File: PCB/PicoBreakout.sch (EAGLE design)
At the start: 41 parts

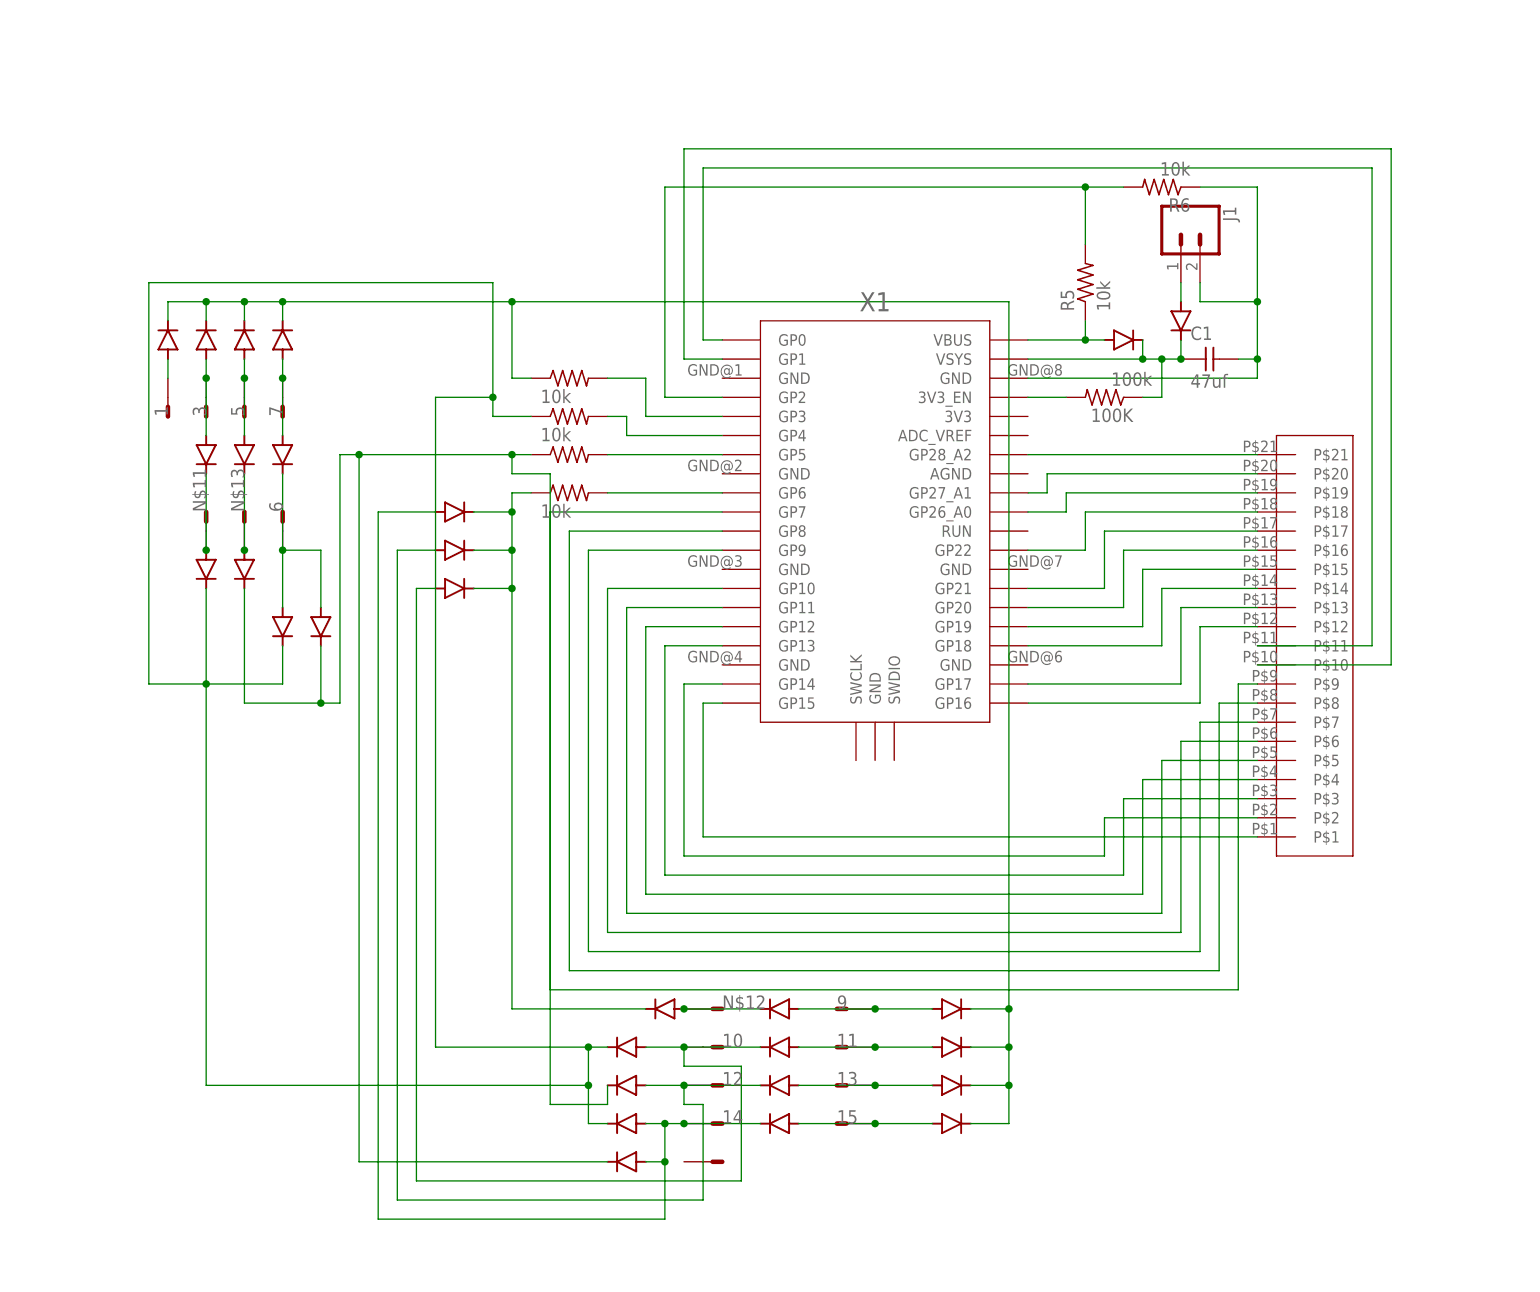
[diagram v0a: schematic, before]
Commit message: schematic push
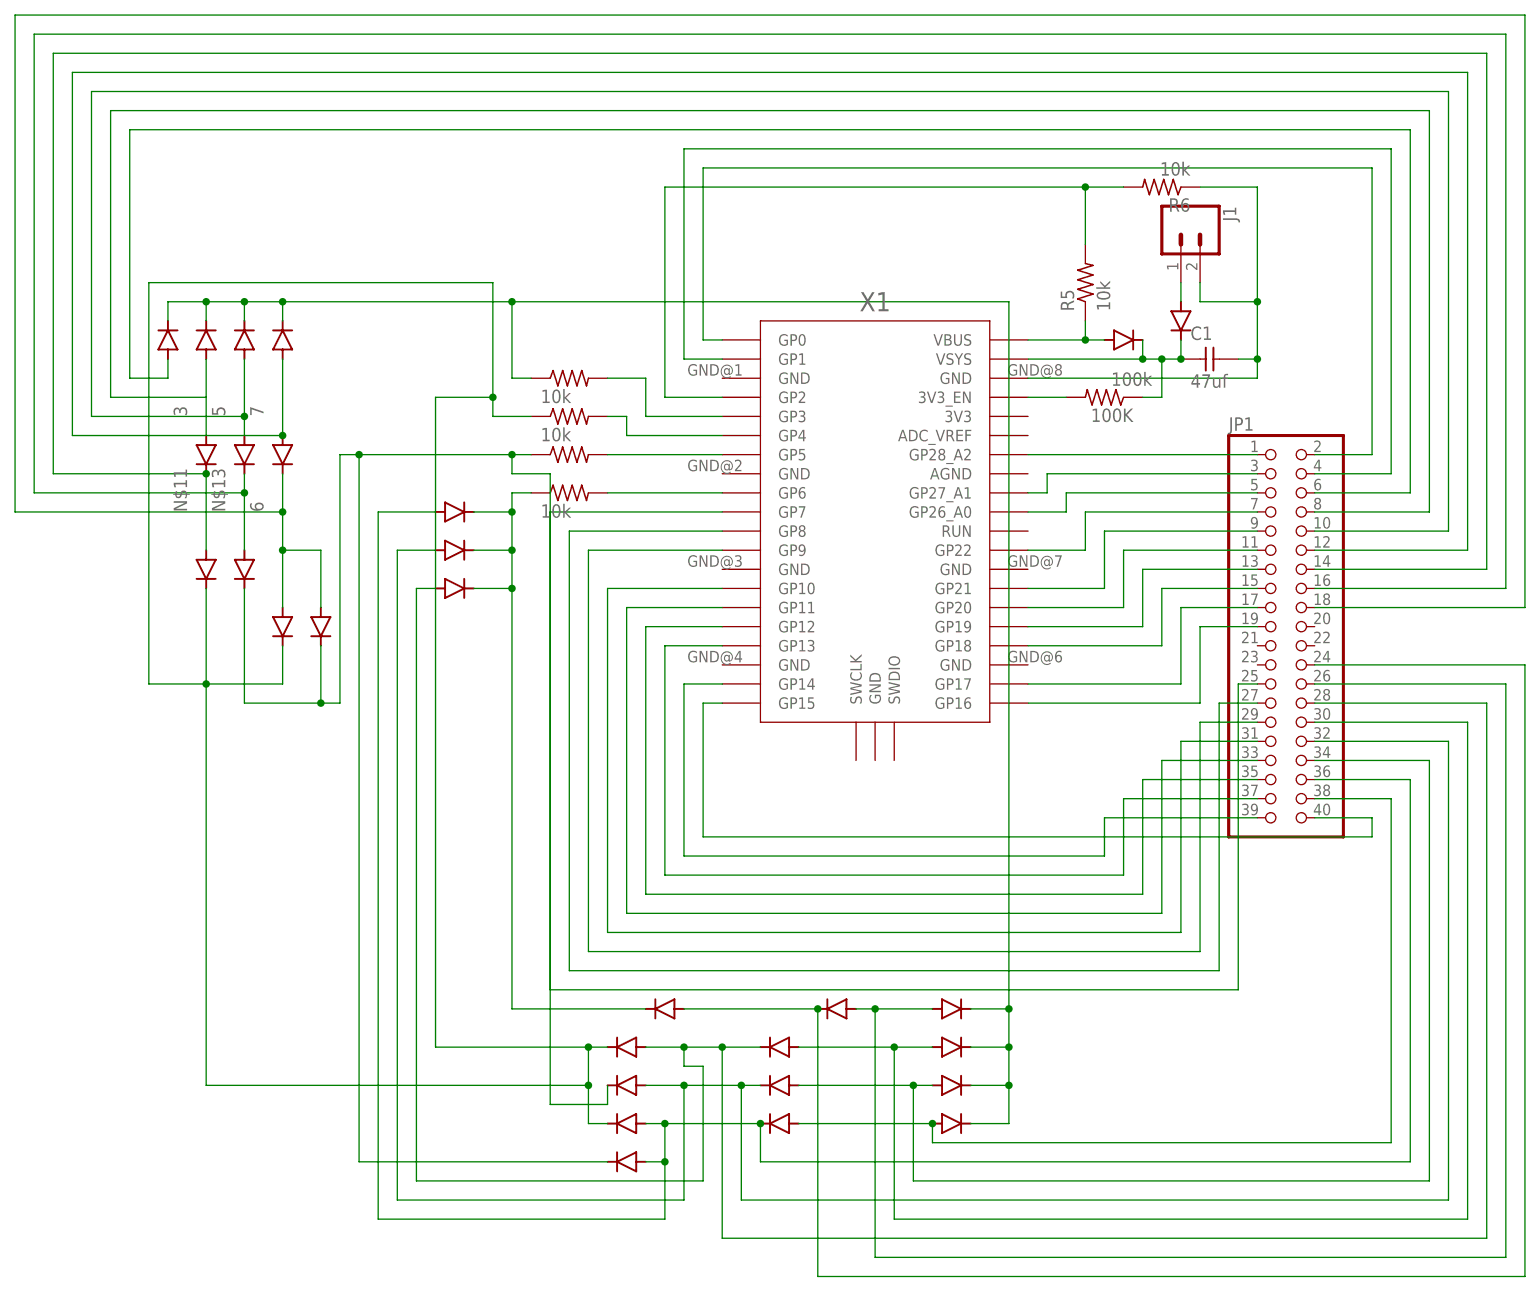
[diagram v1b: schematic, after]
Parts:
- removed SV1: (no value), con-dil:16E
- removed U$1: 21-SMD-CONN, ContunityTestingRig:21-SMD-CONN
- added JP1: (no value), adafruit:PINHD-2X20
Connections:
- net 10: now also JP1.28; no longer SV1-10.S
- net 11: now also JP1.30; no longer SV1-11.S
- net 12: now also JP1.32; no longer SV1-12.S
- net 13: now also JP1.34; no longer SV1-13.S
- net 14: now also JP1.36; no longer SV1-14.S
- net 15: now also JP1.38; no longer SV1-15.S
- net 3: now also JP1.8; no longer SV1-3.S
- net 5: now also JP1.10; no longer SV1-5.S
- net 6: now also JP1.18; no longer SV1-6.S
- net 7: now also JP1.12; no longer SV1-7.S
- net 9: now also JP1.26; no longer SV1-9.S
- net N$10: now also JP1.6; no longer SV1-1.S
- net N$11: now also JP1.14; no longer SV1-2.S
- net N$12: now also JP1.24; no longer SV1-8.S
- net N$13: now also JP1.16; no longer SV1-4.S
- net N$23: now also JP1.1; no longer U$1.P$21
- net N$25: now also JP1.3; no longer U$1.P$20
- net N$26: now also JP1.5; no longer U$1.P$19
- net N$27: now also JP1.7; no longer U$1.P$18
- net N$28: now also JP1.9; no longer U$1.P$17
- net N$29: now also JP1.11; no longer U$1.P$16
- net N$30: now also JP1.13; no longer U$1.P$15
- net N$31: now also JP1.15; no longer U$1.P$14
- net N$32: now also JP1.17; no longer U$1.P$13
- net N$33: now also JP1.19; no longer U$1.P$12
- net N$34: now also JP1.40; no longer U$1.P$1
- net N$35: now also JP1.39; no longer U$1.P$2
- net N$37: now also JP1.35; no longer U$1.P$4
- net N$38: now also JP1.33; no longer U$1.P$5
- net N$39: now also JP1.31; no longer U$1.P$6
- net N$40: now also JP1.29; no longer U$1.P$7
- net N$41: now also JP1.27; no longer U$1.P$8
- net N$42: now also JP1.25; no longer U$1.P$9
- net N$43: now also JP1.2; no longer U$1.P$11
- net N$44: now also JP1.4; no longer U$1.P$10
- net N$48: now also JP1.37; no longer U$1.P$3
